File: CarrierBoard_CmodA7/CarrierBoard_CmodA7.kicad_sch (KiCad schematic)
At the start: 68 parts

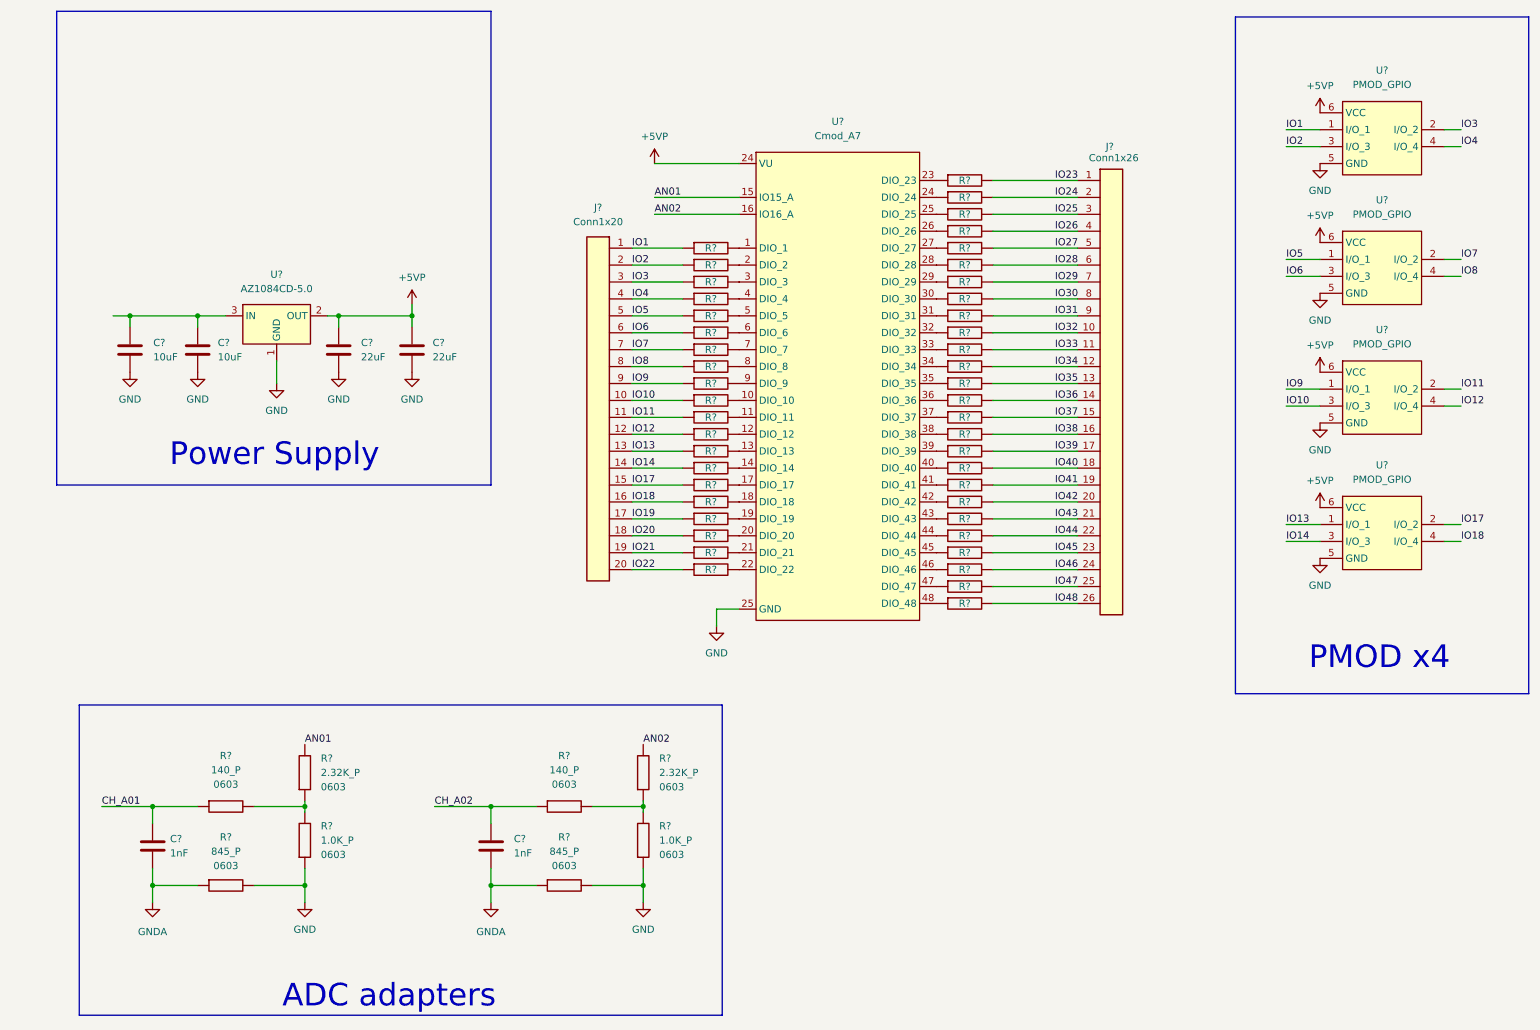
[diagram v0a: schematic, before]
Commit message: Arreglado el circuto del ADC
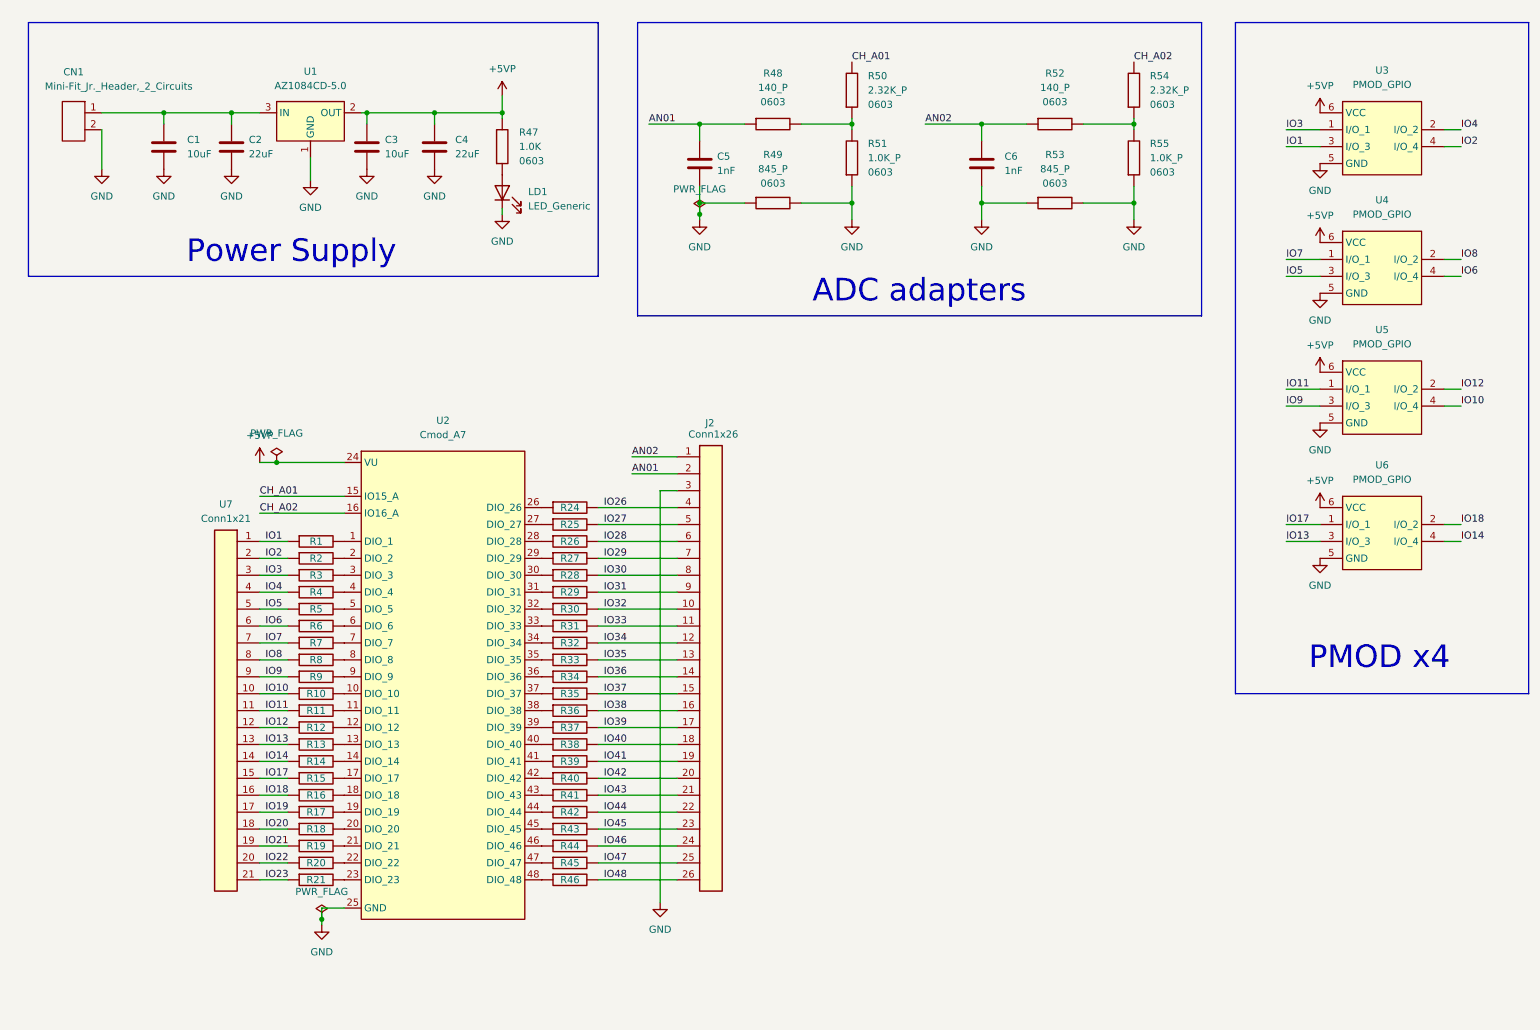
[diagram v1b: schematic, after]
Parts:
- removed C?: 22uF, Capacitor_SMD:C_0805_2012Metric, symbol Herranz - Capacitor (0805):Gen_C
- removed C?: 10uF, Capacitor_SMD:C_0805_2012Metric, symbol Herranz - Capacitor (0805):Gen_C
- removed J?: Conn1x20, Connector_PinHeader_2.54mm:PinHeader_1x20_P2.54mm_Vertical, symbol Herranz - Gen Connectors:Conn1x20
- removed R? (x2): 1.0K, Resistor_SMD:R_0603_1608Metric, symbol Herranz - Resistors (0603):1.0K
- added C2: 22uF, Capacitor_SMD:C_0805_2012Metric, symbol Herranz - Capacitor (0805):Gen_C
- added C3: 10uF, Capacitor_SMD:C_0805_2012Metric, symbol Herranz - Capacitor (0805):Gen_C
- added CN1: Mini-Fit_Jr._Header,_2_Circuits, Herranz - Conn Molex:Mini-Fit Jr. Header, 2 Circuits, symbol Herranz - Conn Molex:Mini-Fit_Jr._Header,_2_Circuits
- added LD1: LED_Generic, LED_SMD:LED_0603_1608Metric_Pad1.05x0.95mm_HandSolder, symbol Herranz - HighpowerLED:LED_Generic
- added R47: 1.0K, Resistor_SMD:R_0603_1608Metric, symbol Herranz - Resistors (0603):1.0K
- added U7: Conn1x21, Connector_PinSocket_2.54mm:PinSocket_1x22_P2.54mm_Vertical, symbol Herranz - Gen Connectors:Conn1x21
- J2: renamed from J?; footprint Connector_PinHeader_2.54mm:PinHeader_1x26_P2.54mm_Vertical -> Connector_PinSocket_2.54mm:PinSocket_1x26_P2.54mm_Vertical
- U2: renamed from U?; footprint (none) -> Herranz - DevBoards:CmodA7
- U3, U4, U5, U6: renamed from U?; footprint Connector_PinHeader_2.54mm:PinHeader_2x03_P2.54mm_Horizontal -> Connector_PinSocket_2.54mm:PinSocket_2x03_P2.54mm_Horizontal
- gave numbers to parts that had none: 57
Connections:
- net GNDA is gone; now on net GND: C5.2, C6.2, R49.1, R53.1
- net IO24 is gone; now on net AN01: J2.2 (Pin_2)
- net IO25 is gone; now on net GND: J2.3 (Pin_3)
- net +5VP: now also C3.1, R47.2
- net AN01: now also C5.1, R48.1; no longer R50.2, U2.15 (IO15_A)
- net AN02: now also C6.1, J2.1 (Pin_1), R52.1; no longer R54.2, U2.16 (IO16_A)
- net CH_A01: now also R50.2, U2.15 (IO15_A); no longer C5.1, R48.1
- net CH_A02: now also R54.2, U2.16 (IO16_A); no longer C6.1, R52.1
- net GND: now also C2.2, C3.2, CN1.2, LD1.2 (K)
- net IO1: now also U3.3 (I/O_3), U7.1 (Pin_1); no longer U3.1 (I/O_1)
- net IO10: now also U5.4 (I/O_4), U7.10 (Pin_10); no longer U5.3 (I/O_3)
- net IO11: now also U5.1 (I/O_1), U7.11 (Pin_11); no longer U5.2 (I/O_2)
- net IO12: now also U5.2 (I/O_2), U7.12 (Pin_12); no longer U5.4 (I/O_4)
- net IO13: now also U6.3 (I/O_3), U7.13 (Pin_13); no longer U6.1 (I/O_1)
- net IO14: now also U6.4 (I/O_4), U7.14 (Pin_14); no longer U6.3 (I/O_3)
- net IO17: now also U6.1 (I/O_1), U7.15 (Pin_15); no longer U6.2 (I/O_2)
- net IO18: now also U6.2 (I/O_2), U7.16 (Pin_16); no longer U6.4 (I/O_4)
- net IO19: now also U7.17 (Pin_17)
- net IO2: now also U3.4 (I/O_4), U7.2 (Pin_2); no longer U3.3 (I/O_3)
- net IO20: now also U7.18 (Pin_18)
- net IO21: now also U7.19 (Pin_19)
- net IO22: now also U7.20 (Pin_20)
- net IO23: now also R21.1, U7.21 (Pin_21); no longer J2.1 (Pin_1), R21.2
- net IO3: now also U3.1 (I/O_1), U7.3 (Pin_3); no longer U3.2 (I/O_2)
- net IO4: now also U3.2 (I/O_2), U7.4 (Pin_4); no longer U3.4 (I/O_4)
- net IO5: now also U4.3 (I/O_3), U7.5 (Pin_5); no longer U4.1 (I/O_1)
- net IO6: now also U4.4 (I/O_4), U7.6 (Pin_6); no longer U4.3 (I/O_3)
- net IO7: now also U4.1 (I/O_1), U7.7 (Pin_7); no longer U4.2 (I/O_2)
- net IO8: now also U4.2 (I/O_2), U7.8 (Pin_8); no longer U4.4 (I/O_4)
- net IO9: now also U5.3 (I/O_3), U7.9 (Pin_9); no longer U5.1 (I/O_1)
- net at C1.1, U1.3 (IN): now also C2.1, CN1.1
- net at U2.23 (DIO_23): now also R21.2; no longer R21.1
- new net: LD1.1 (A), R47.1
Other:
- moved on the sheet: C1, C4, C5, C6, J2, R1, R10, R11, R12, R13, R14, R15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
